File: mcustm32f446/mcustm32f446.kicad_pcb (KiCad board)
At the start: 2 copper layers, 76.2 x 50.8 mm, 34 parts, among them J2 STM32WORLD_BASE, U1 AMS1117-3.3, U2 SRV05-4, U3 STM32F446RCTx, Y1 X_16MHZ

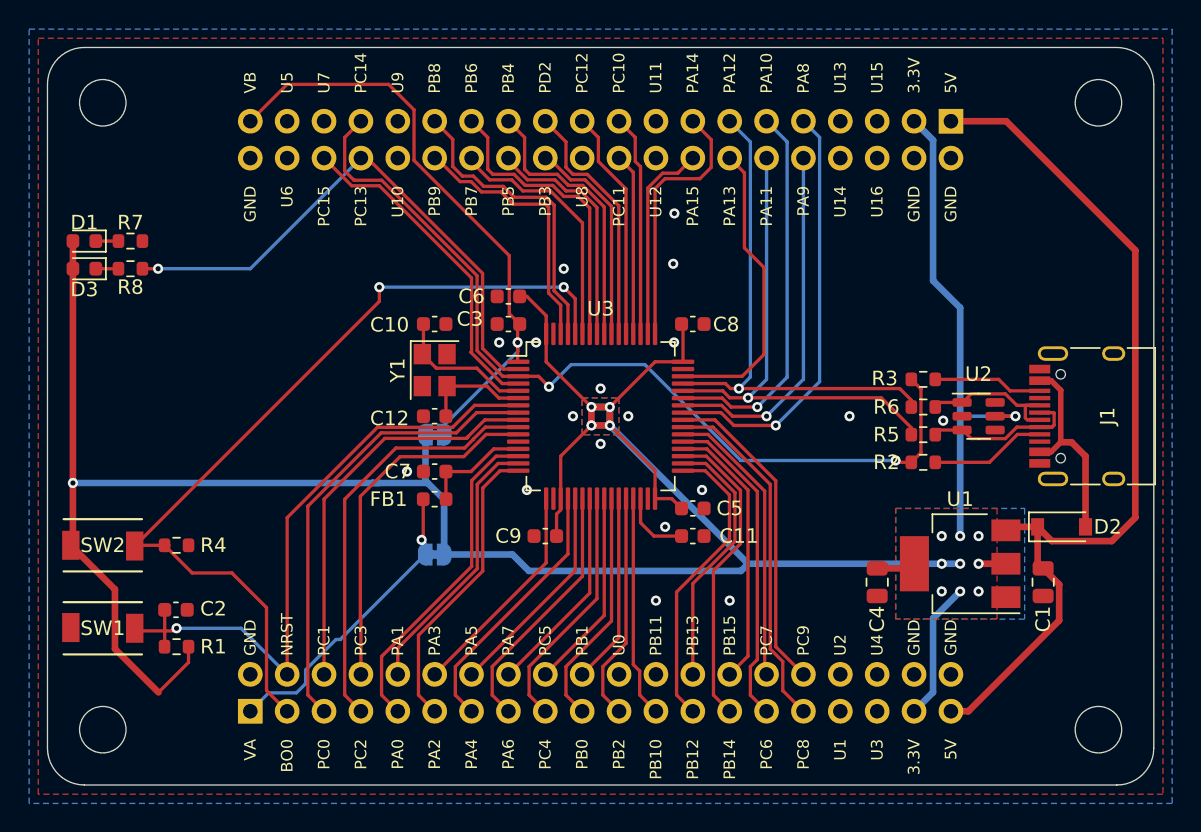
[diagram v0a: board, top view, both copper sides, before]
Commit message: Hmmm
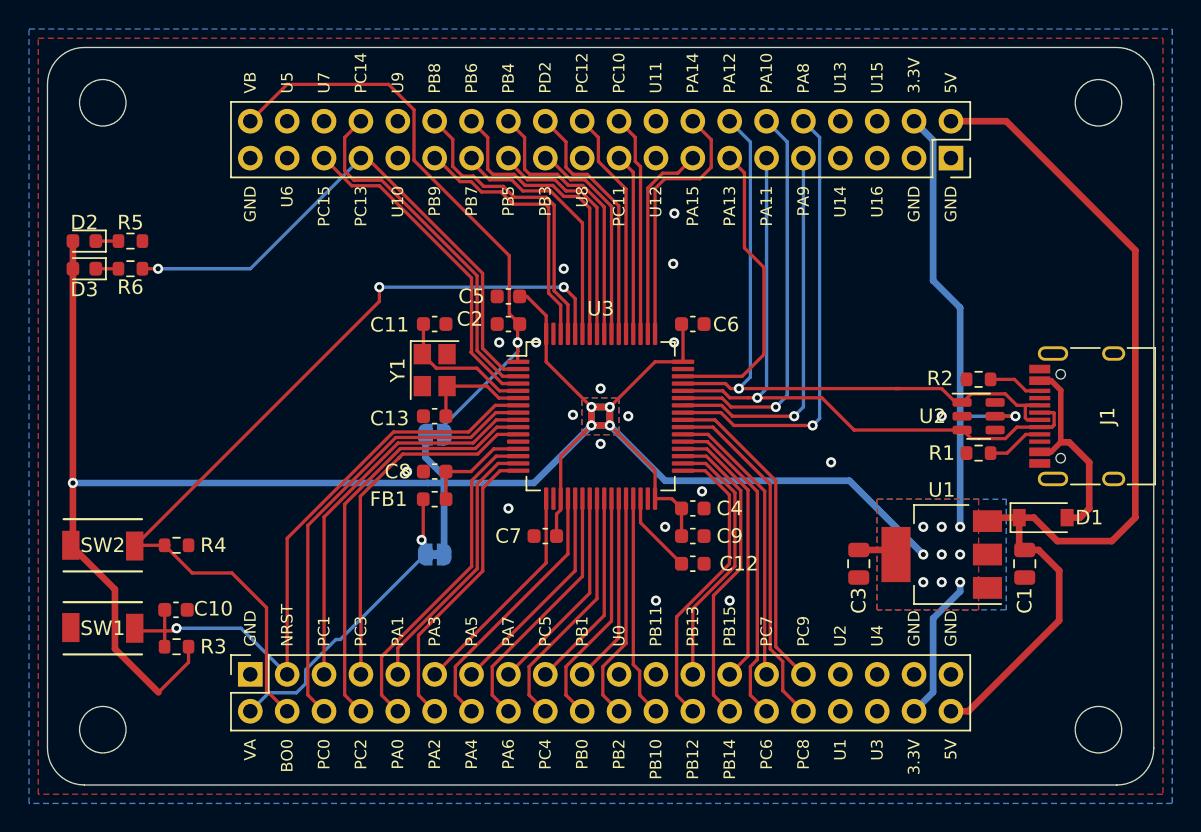
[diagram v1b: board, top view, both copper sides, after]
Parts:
- removed the R5 at (174.6, 102.9)
- removed the R6 at (174.6, 101.0)
- added C9: C_100NF_0603, Capacitor_SMD:C_0603_1608Metric, F.Cu at (158.8, 109.9)
- added J3: STM32WORLD_CONNECTOR_2, stm32world:PinSocket_2x20_P2.54mm_Vertical_Stackable, F.Cu at (176.5, 83.8)
- added J4: STM32WORLD_BOARD, stm32world:STM32WORLD_BOARD, F.Cu at (152.4, 101.6)
- J2: value STM32WORLD_BASE -> STM32WORLD_CONNECTOR_1; footprint stm32world:STM32WORLD_BASE -> stm32world:PinSocket_2x20_P2.54mm_Vertical_Stackable
- moved J2 30.0 mm to (128.3, 119.4), turned to 90 degrees
- moved R1 3.86 mm to (178.4, 104.1)
- moved R2 3.81 mm to (178.4, 99.1)
- moved C12 1.91 mm to (158.8, 111.8)
- moved C1 1.80 mm to (181.6, 111.8)
- moved C3 1.80 mm to (170.2, 111.8)
- moved D1 1.42 mm to (182.9, 108.6)
- moved U1 1.42 mm to (175.9, 111.1)
- renumbered C2 to C10, C10 to C11, C11 to C12, C12 to C13, C3 to C2, C4 to C3, C5 to C4, C6 to C5, C8 to C6, C9 to C7, C7 to C8, D2 to D1, D1 to D2, R2 to R1, R3 to R2, R1 to R3, R7 to R5, R8 to R6
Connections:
- J1 pad A6: Net-(J1-PadA6) -> PA12
- J1 pad A7: Net-(J1-PadA7) -> PA11
- J1 pad B6: Net-(J1-PadA6) -> PA12
- J1 pad B7: Net-(J1-PadA7) -> PA11
- J2 pad 1: VA -> GND
- J2 pad 10: PA1 -> PA0
- J2 pad 11: PA2 -> PA3
- J2 pad 12: PA3 -> PA2
- J2 pad 13: PA4 -> PA5
- J2 pad 14: PA5 -> PA4
- J2 pad 15: PA6 -> PA7
- J2 pad 16: PA7 -> PA6
- J2 pad 17: PC4 -> PC5
- J2 pad 18: PC5 -> PC4
- J2 pad 19: PB0 -> PB1
- J2 pad 2: GND -> VA
- J2 pad 20: PB1 -> PB0
- J2 pad 21: PB2 -> unconnected-(J2-Pad21)
- J2 pad 22: unconnected-(J2-Pad22) -> PB2
- J2 pad 23: PB10 -> unconnected-(J2-Pad23)
- J2 pad 24: unconnected-(J2-Pad24) -> PB10
- J2 pad 25: PB12 -> PB13
- J2 pad 26: PB13 -> PB12
- J2 pad 27: PB14 -> PB15
- J2 pad 28: PB15 -> PB14
- J2 pad 29: PC6 -> PC7
- J2 pad 3: BO0 -> NRST
- J2 pad 30: PC7 -> PC6
- J2 pad 31: PC8 -> PC9
- J2 pad 32: PC9 -> PC8
- J2 pad 37: +3V3 -> GND
- J2 pad 38: GND -> +3V3
- J2 pad 39: +5V -> GND
- J2 pad 4: NRST -> BO0
- J2 pad 40: GND -> +5V
- J2 pad 5: PC0 -> PC1
- J2 pad 6: PC1 -> PC0
- J2 pad 7: PC2 -> PC3
- J2 pad 8: PC3 -> PC2
- J2 pad 9: PA0 -> PA1
- R1 pad 1: PC14 -> GND
- R2 pad 1: PC14 -> GND
- U2 pad 1: Net-(J1-PadA6) -> PA12
- U2 pad 3: Net-(J1-PadA7) -> PA11
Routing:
- net PC14: track 61.8 -> 24.7 mm, vias 2 -> 0
- net PA12: track 36.0 -> 48.1 mm
- net PA11: track 34.3 -> 45.9 mm
- net +3V3: track 215.7 -> 204.2 mm
- net Net-(J1-PadA7): track 10.8 -> 0.00 mm
- net Net-(J1-PadA6): track 10.8 -> 0.00 mm
- net Net-(J1-PadA5): track 7.99 -> 3.92 mm
- net Net-(J1-PadB5): track 7.52 -> 3.71 mm
- net +5V: track 61.7 -> 65.2 mm
- net PA8: track 29.4 -> 30.9 mm
- net PA9: track 24.9 -> 26.0 mm
- net NRST: track 44.2 -> 43.3 mm
- net Net-(C12-Pad1): track 4.87 -> 5.66 mm
- net PC0: track 31.7 -> 31.0 mm
- net PA10: track 26.5 -> 27.2 mm
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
